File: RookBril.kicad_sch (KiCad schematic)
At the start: 26 parts, among them J1 IR_SENSOR0_PINS, J2 IR_SENSOR2_PINS, J3 IR_SENSOR1_PINS, J4 IR_SENSOR2_PINS, J6 PDLC_JST_PINS, J7 PROGRAM_PINS, SW1 SW_Push, U1 VNH7070ASTR, U2 STM32F411RETx

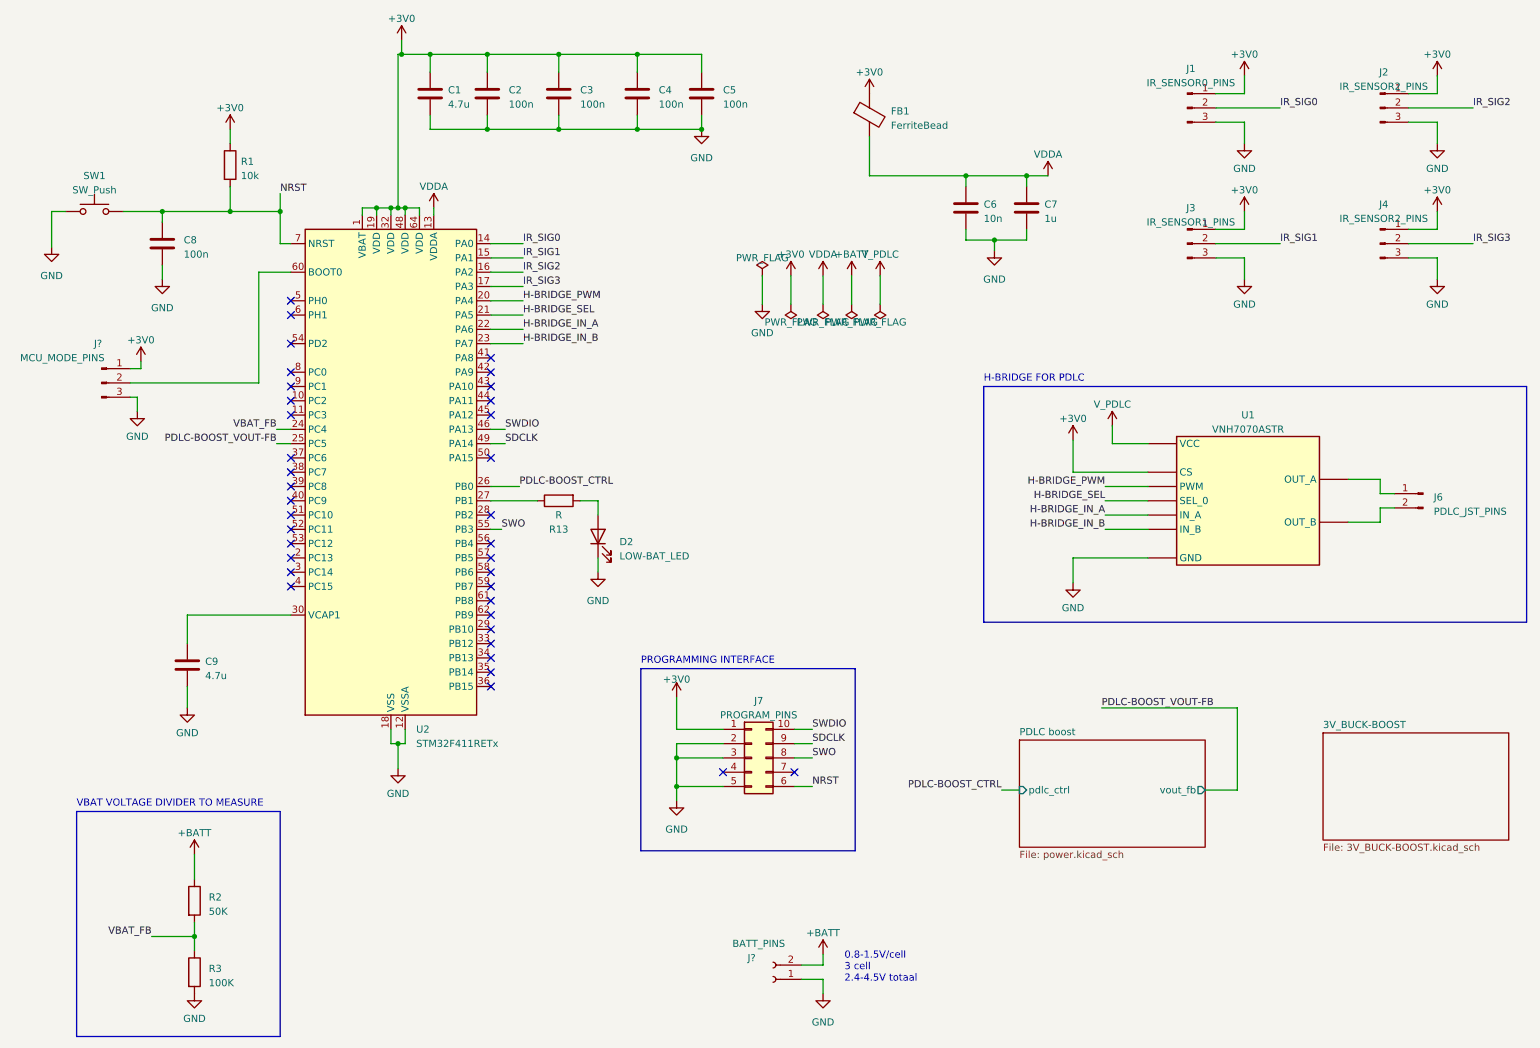
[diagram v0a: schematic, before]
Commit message: footprint assignments gedaan + verbeteringen
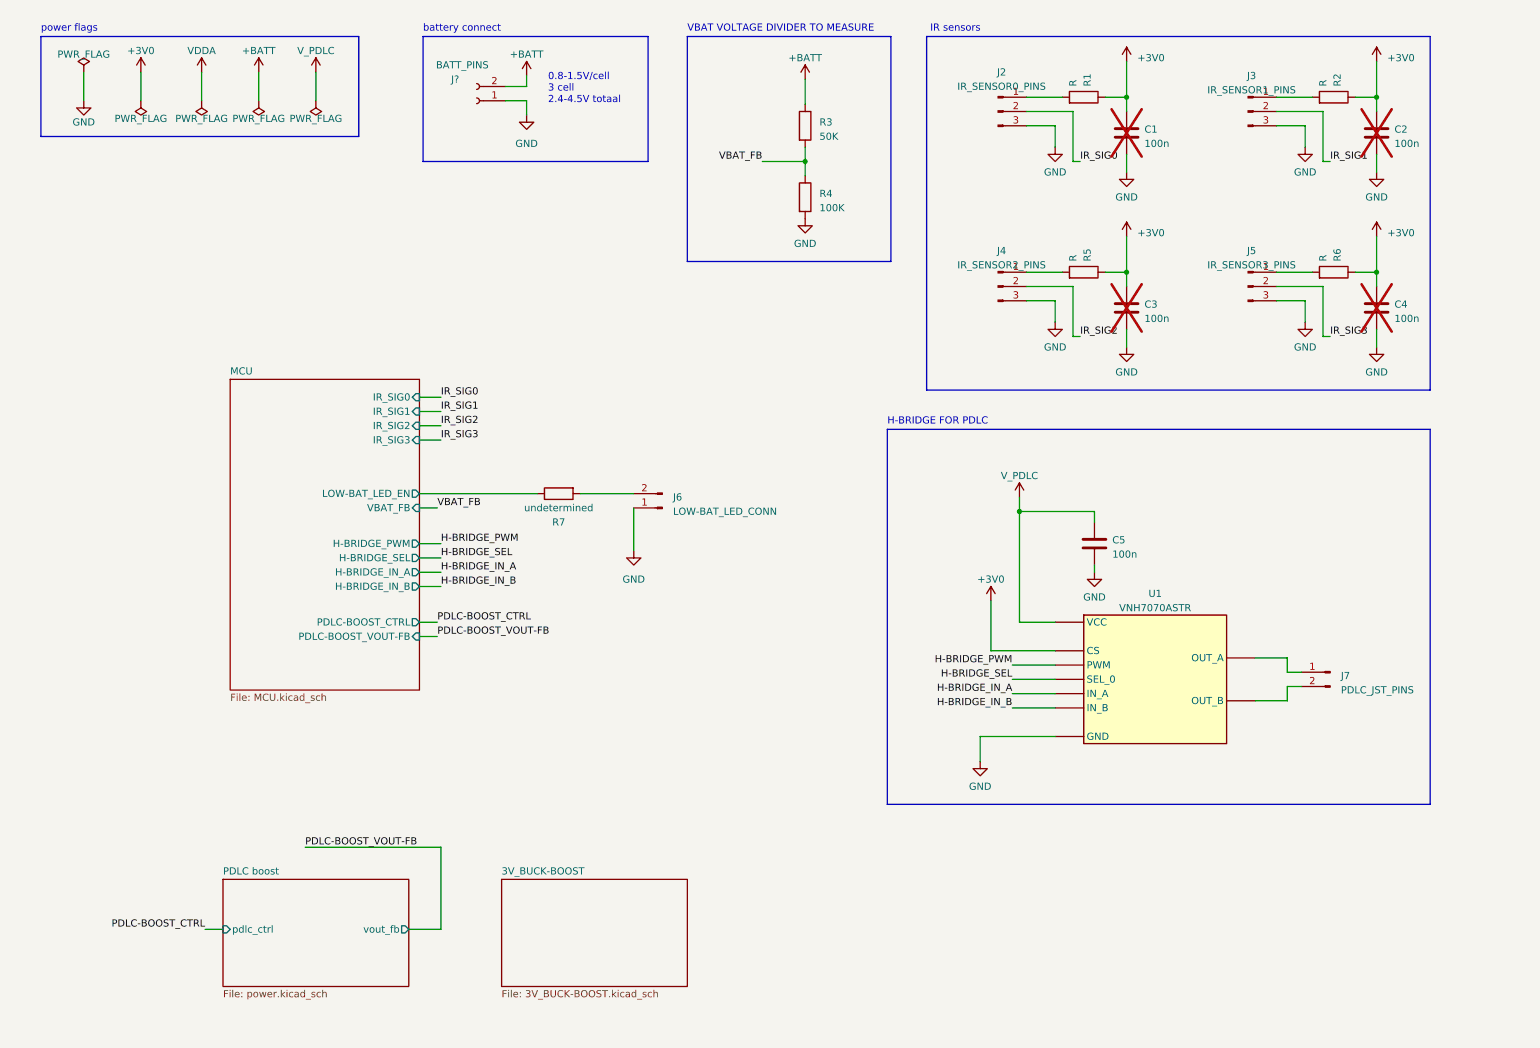
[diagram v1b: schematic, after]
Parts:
- removed C6: 10n, symbol Device:C
- removed C7: 1u, symbol Device:C
- removed C8: 100n, symbol Device:C
- removed C9: 4.7u, symbol Device:C
- removed D2: LOW-BAT_LED, symbol Device:LED
- removed FB1: FerriteBead, symbol Device:FerriteBead
- removed J2: IR_SENSOR2_PINS, symbol Connector:Conn_01x03_Pin
- removed J7: PROGRAM_PINS, symbol Connector_Generic:Conn_02x05_Counter_Clockwise
- removed J?: MCU_MODE_PINS, symbol Connector:Conn_01x03_Pin
- removed SW1: SW_Push, symbol Switch:SW_Push
- removed U2: STM32F411RETx, Package_QFP:LQFP-64_10x10mm_P0.5mm, symbol MCU_ST_STM32F4:STM32F411RETx
- added J5: IR_SENSOR3_PINS, Connector_PinHeader_2.54mm:PinHeader_1x03_P2.54mm_Vertical, symbol Connector:Conn_01x03_Pin
- added J6: LOW-BAT_LED_CONN, Connector_PinHeader_2.54mm:PinHeader_1x02_P2.54mm_Vertical, symbol Connector:Conn_01x02_Pin
- added R2, R5, R6: R, Resistor_SMD:R_0805_2012Metric_Pad1.20x1.40mm_HandSolder, symbol Device:R
- C1: value 4.7u -> 100n; footprint (none) -> Capacitor_SMD:C_0805_2012Metric_Pad1.18x1.45mm_HandSolder; now not fitted
- C2, C3, C4: footprint (none) -> Capacitor_SMD:C_0805_2012Metric_Pad1.18x1.45mm_HandSolder; now not fitted
- C5: footprint (none) -> Capacitor_SMD:C_0805_2012Metric_Pad1.18x1.45mm_HandSolder
- J2: renamed from J1; footprint (none) -> Connector_PinHeader_2.54mm:PinHeader_1x03_P2.54mm_Vertical
- J3, J4: footprint (none) -> Connector_PinHeader_2.54mm:PinHeader_1x03_P2.54mm_Vertical
- J7: renamed from J6; footprint (none) -> Connector_PinHeader_2.54mm:PinHeader_1x02_P2.54mm_Vertical
- J?: footprint (none) -> Connector_PinHeader_2.54mm:PinHeader_1x02_P2.54mm_Vertical
- R1: value 10k -> R; footprint (none) -> Resistor_SMD:R_0805_2012Metric_Pad1.20x1.40mm_HandSolder
- R3: renamed from R2; footprint (none) -> Resistor_SMD:R_0805_2012Metric_Pad1.20x1.40mm_HandSolder
- R4: renamed from R3; footprint (none) -> Resistor_SMD:R_0805_2012Metric_Pad1.20x1.40mm_HandSolder
- R7: renamed from R13; value R -> undetermined; footprint (none) -> Resistor_SMD:R_0805_2012Metric_Pad1.20x1.40mm_HandSolder
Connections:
- net +3V0: now also R2.1, R5.1, R6.1; no longer C5.1, J2.1 (Pin_1), J3.1 (Pin_1), J4.1 (Pin_1)
- net GND: now also J5.3 (Pin_3), J6.1 (Pin_1)
- net IR_SIG2: now also J4.2 (Pin_2)
- net IR_SIG3: now also J5.2 (Pin_2); no longer J4.2 (Pin_2)
- net VCC: now also C5.1
- net MCU/LOW-BAT_LED_EN: now reaches R7.1
- net at R7.2: now also J6.2 (Pin_2)
- net NRST: no longer names the net of R1.2
- net NRST: now also J2.1 (Pin_1)
- new net: J4.1 (Pin_1), R5.2
- new net: J3.1 (Pin_1), R2.2
- new net: J5.1 (Pin_1), R6.2
- no-connect marks 37 -> 0
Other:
- added sheet MCU (MCU.kicad_sch)
- note added: "IR sensors"
- note added: "battery connect"
- note added: "power flags"
- note removed: "PROGRAMMING INTERFACE"
- moved on the sheet: J2, J7, J?, R3, R4, R7, U1
